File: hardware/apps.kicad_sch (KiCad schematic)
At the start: 22 parts, among them SW1 SW_Push, U1 STM32L4P5RET6, Y1 8Mhz

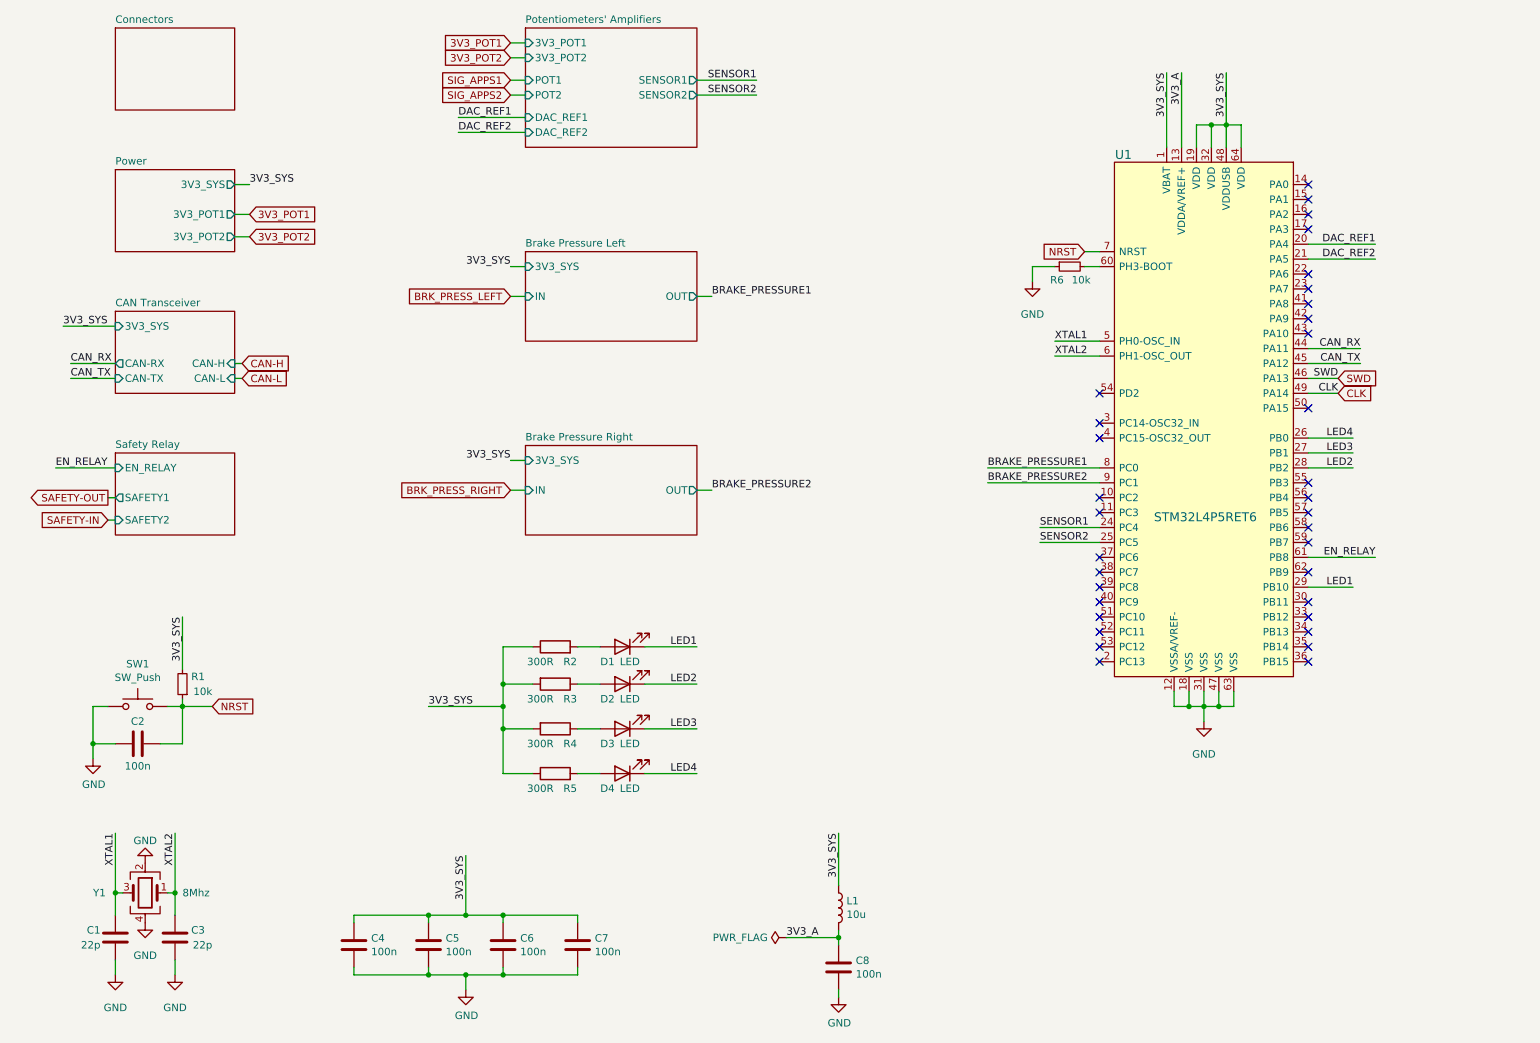
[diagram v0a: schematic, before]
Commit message: Refactor
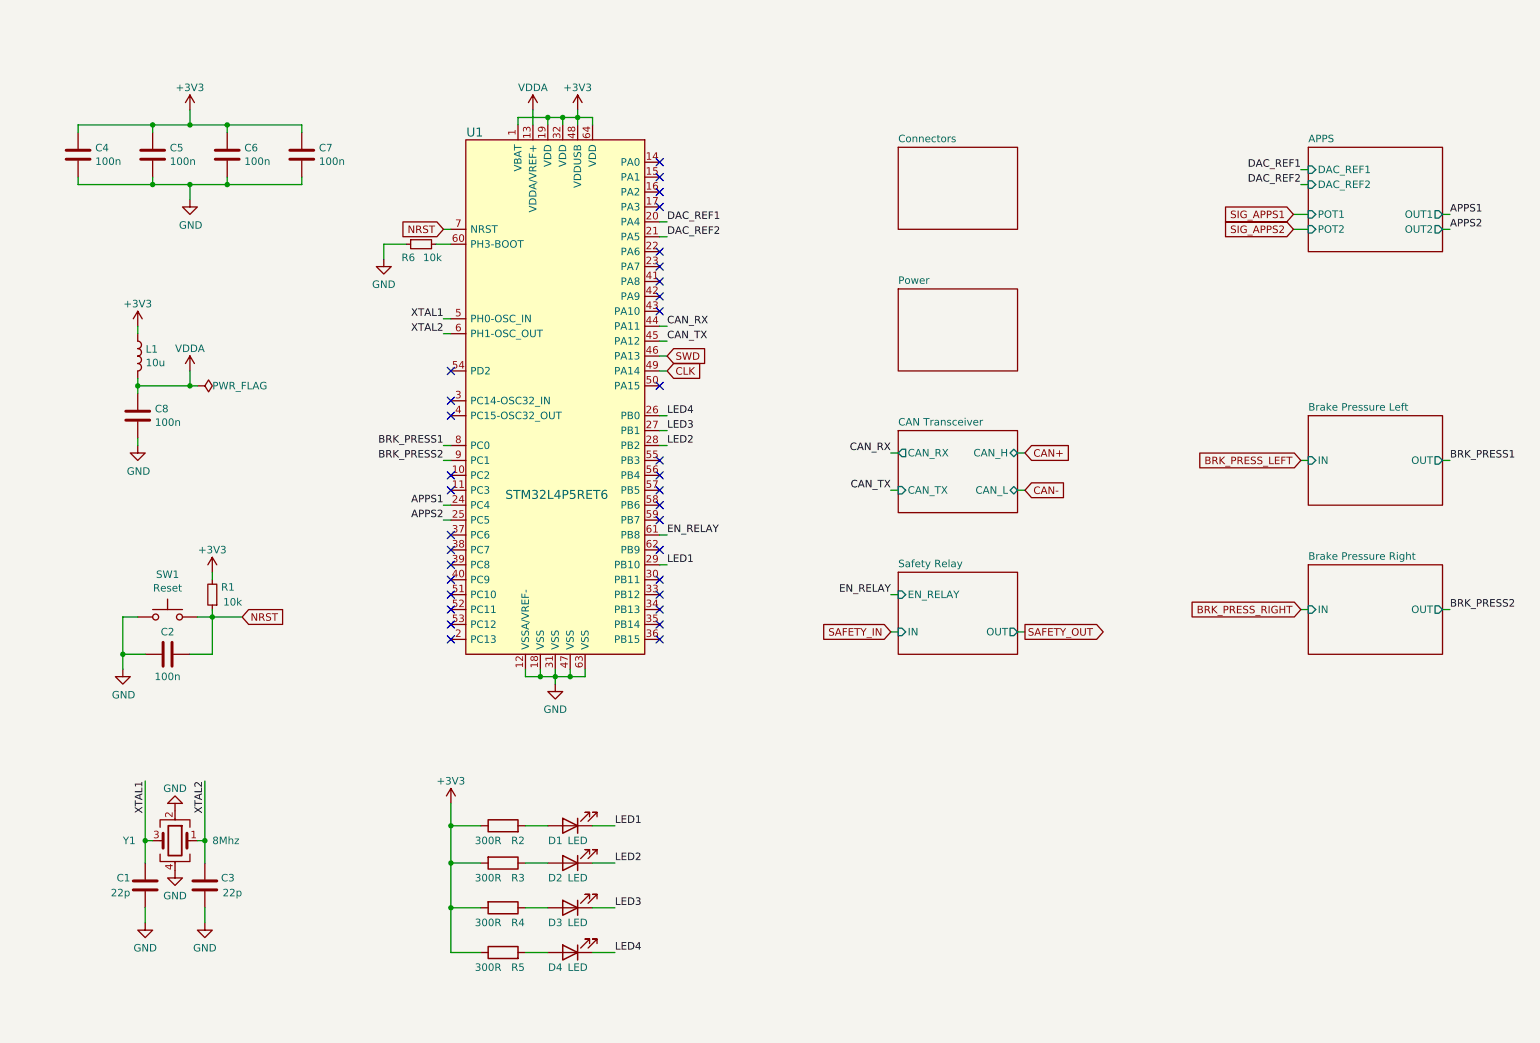
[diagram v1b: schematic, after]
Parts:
- SW1: value SW_Push -> Reset
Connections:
- net 3V3_A renamed VDDA
- net 3V3_SYS renamed +3V3
- net BRAKE_PRESSURE1 renamed BRK_PRESS1
- net BRAKE_PRESSURE2 renamed BRK_PRESS2
- net SENSOR1 renamed APPS1
- net SENSOR2 renamed APPS2
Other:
- sheet Potentiometers' Amplifiers renamed APPS
- sheet APPS: file AnalogInputs.kicad_sch -> analog_inputs.kicad_sch
- sheet APPS ports: added OUT1, OUT2; removed 3V3_POT1, 3V3_POT2, SENSOR1, SENSOR2
- sheet Brake Pressure Left ports: added none; removed 3V3_SYS
- sheet Brake Pressure Right ports: added none; removed 3V3_SYS
- sheet CAN Transceiver: file CAN.kicad_sch -> can_transceiver.kicad_sch
- sheet CAN Transceiver ports: added CAN_H, CAN_L, CAN_RX, CAN_TX; removed 3V3_SYS, CAN-H, CAN-L, CAN-RX, CAN-TX
- sheet Connectors: file Connectros.kicad_sch -> connectors.kicad_sch
- sheet Power: file PowerModule.kicad_sch -> power_module.kicad_sch
- sheet Power ports: added none; removed 3V3_POT1, 3V3_POT2, 3V3_SYS
- sheet Safety Relay: file Safety.kicad_sch -> safety_relay.kicad_sch
- sheet Safety Relay ports: added IN, OUT; removed SAFETY1, SAFETY2
- moved on the sheet: C1, C2, C3, C4, C5, C6, C7, C8, D1, D2, D3, D4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
